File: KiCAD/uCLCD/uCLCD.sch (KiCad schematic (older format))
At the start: 18 parts, among them IC1 ATMEGA328P-P, P1 CONN_01X12, P2 CONN_01X03, P3 CONN_01X03, P4 CONN_01X03, P5 CONN_01X02, P6 CONN_01X03, P7 p_button, P8 p_button, P9 p_button, U1 DDS, Y1 16Mhz

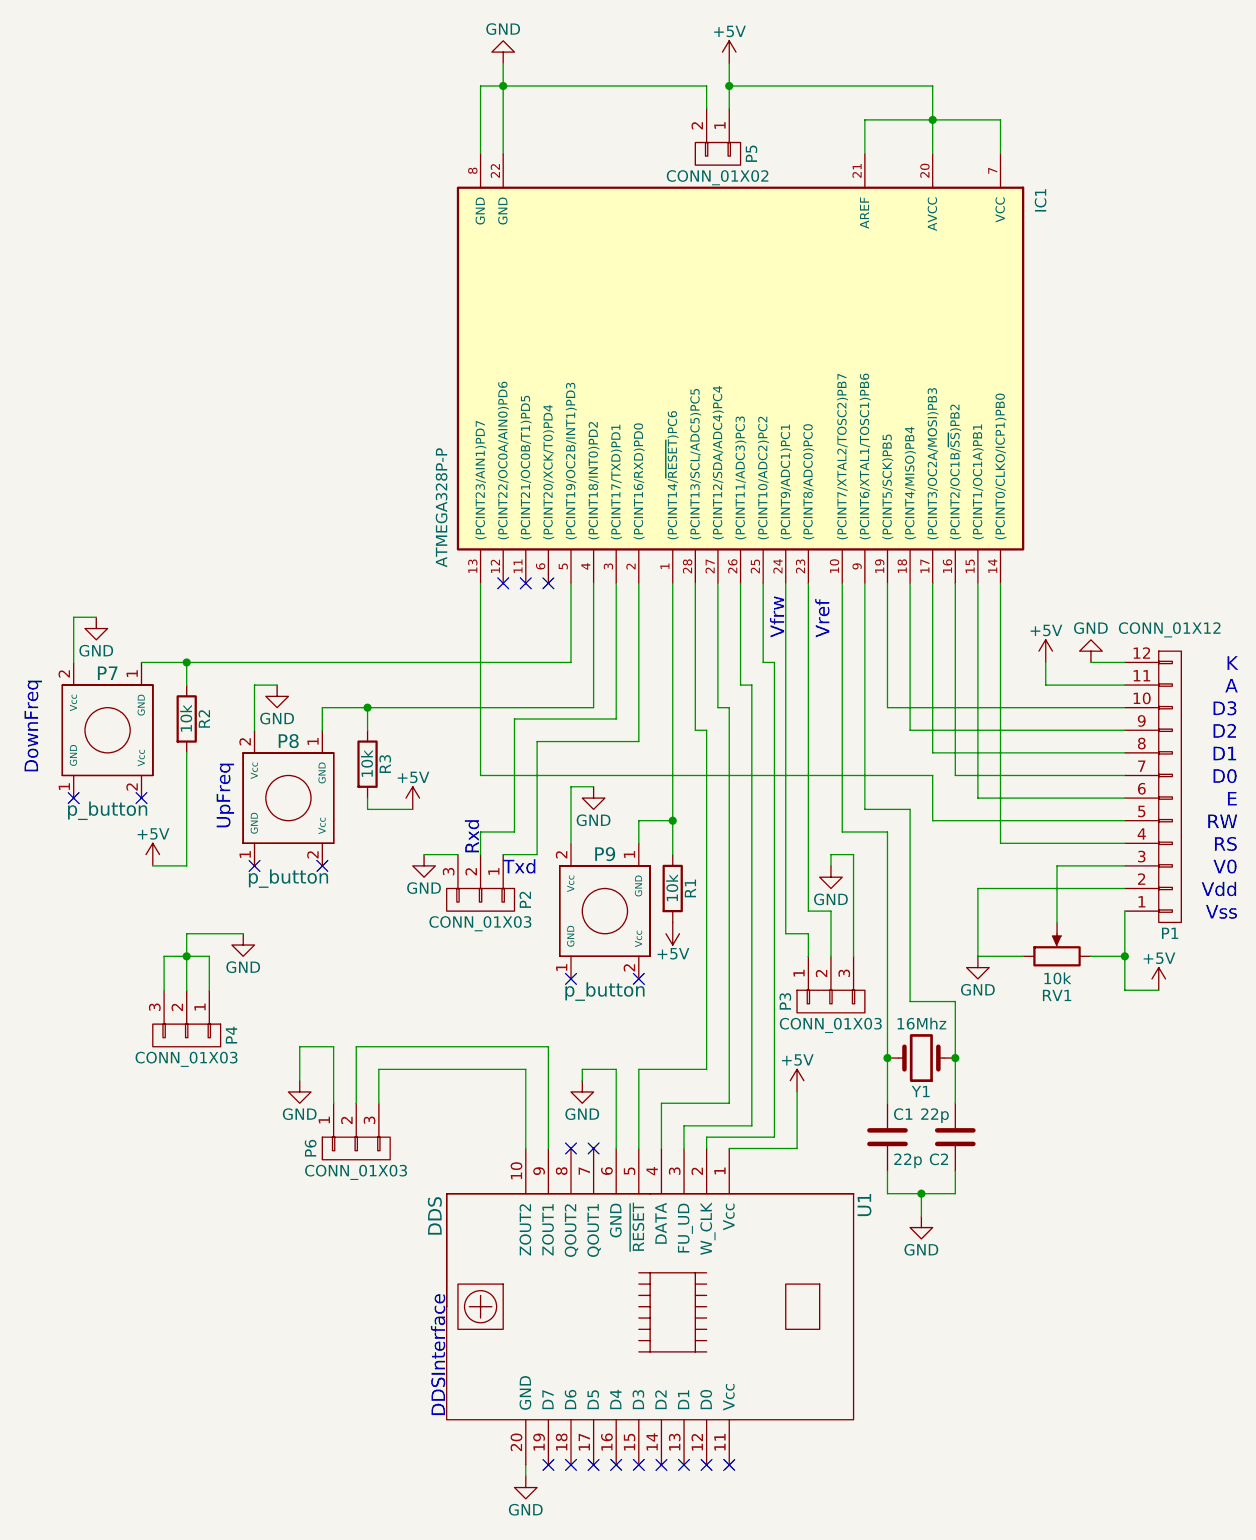
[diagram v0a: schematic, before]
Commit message: latest changes
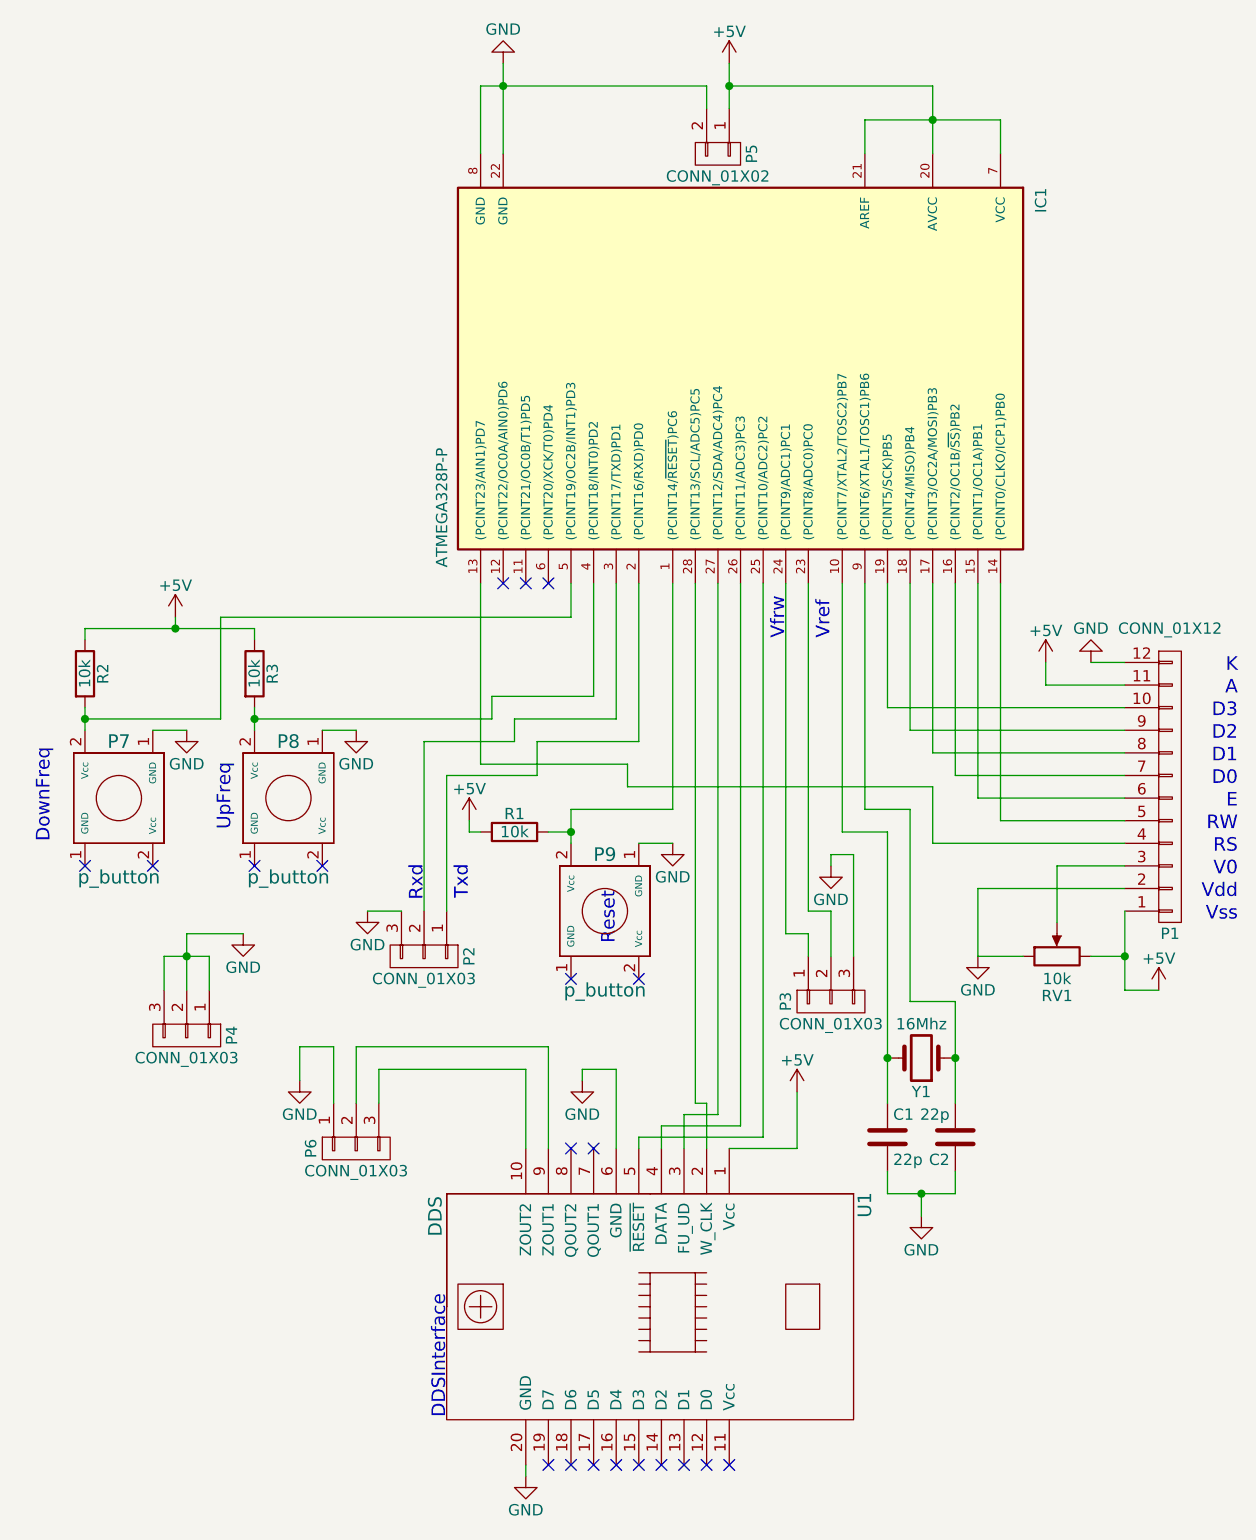
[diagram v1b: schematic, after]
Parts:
- P7, P8, P9: footprint uCLCD:p_button -> Buttons_Switches_ThroughHole:SW_PUSH_6mm_h7.3mm
- R1, R2, R3: footprint Resistors_ThroughHole:Resistor_Horizontal_RM7mm -> Resistors_THT:R_Axial_DIN0207_L6.3mm_D2.5mm_P10.16mm_Horizontal
- RV1: footprint Potentiometers:Potentiometer_VishaySpectrol_248GJ_249GJ_Vertical -> Potentiometers:Potentiometer_Trimmer_ACP_CA6v_Horizontal
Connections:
- net +5V: now also R1.1, R2.1, R3.1; no longer R1.2, R2.2, R3.2
- net GND: now also P7.1 (GND), P8.1 (GND), P9.1 (GND); no longer P7.2 (Vcc), P8.2 (Vcc), P9.2 (Vcc)
- net at IC1.13 ((PCINT23/AIN1)PD7): now also P1.4 (P4); no longer P1.5 (P5)
- net at IC1.14 ((PCINT0/CLKO/ICP1)PB0): now also P1.5 (P5); no longer P1.4 (P4)
- net at IC1.25 ((PCINT10/ADC2)PC2): now also U1.5 (~RESET); no longer U1.2 (W_CLK)
- net at IC1.26 ((PCINT11/ADC3)PC3): now also U1.4 (DATA); no longer U1.3 (FU_UD)
- net at IC1.27 ((PCINT12/SDA/ADC4)PC4): now also U1.3 (FU_UD); no longer U1.4 (DATA)
- net at IC1.28 ((PCINT13/SCL/ADC5)PC5): now also U1.2 (W_CLK); no longer U1.5 (~RESET)
- new net: IC1.1 ((PCINT14/~RESET~)PC6), P9.2 (Vcc), R1.2
- new net: IC1.4 ((PCINT18/INT0)PD2), P8.2 (Vcc), R3.2
- new net: IC1.5 ((PCINT19/OC2B/INT1)PD3), P7.2 (Vcc), R2.2
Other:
- note added: "Reset"
- moved on the sheet: P2, P7, R1, R2, R3
